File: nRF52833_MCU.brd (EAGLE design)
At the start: 51.3 x 30.2 mm, 64 parts, among them IC1 SKY13415-485LF, J1 282834-2, J100 DEBUG_CONNECTOR, J2 282834-2, J3 282834-2, U1 nRF52833-QIAA, U3 BQ25570RGRR, X1 32MHz, X2 32.768kHz, X3 22-23-2031

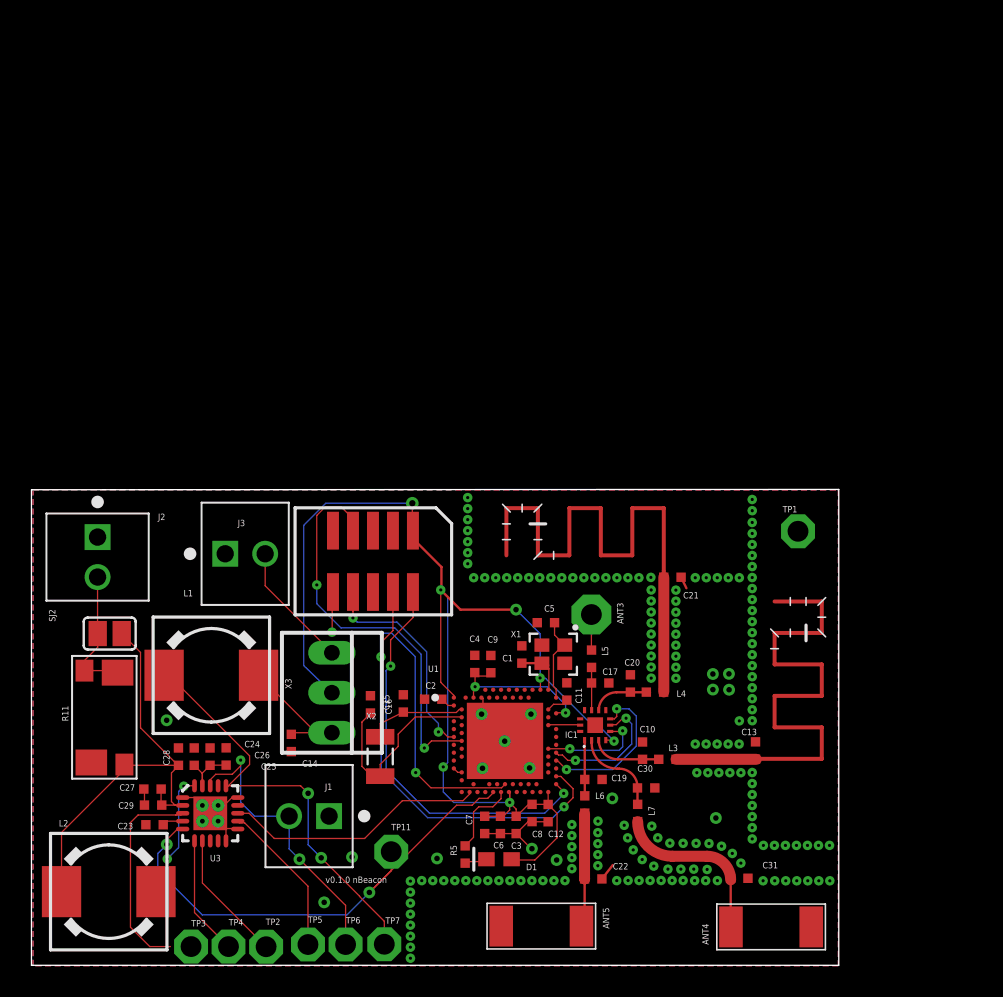
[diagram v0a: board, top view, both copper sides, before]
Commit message: Fix warnings
Signed-off-by: Florian Depraz <florian.depraz@outlook.com>
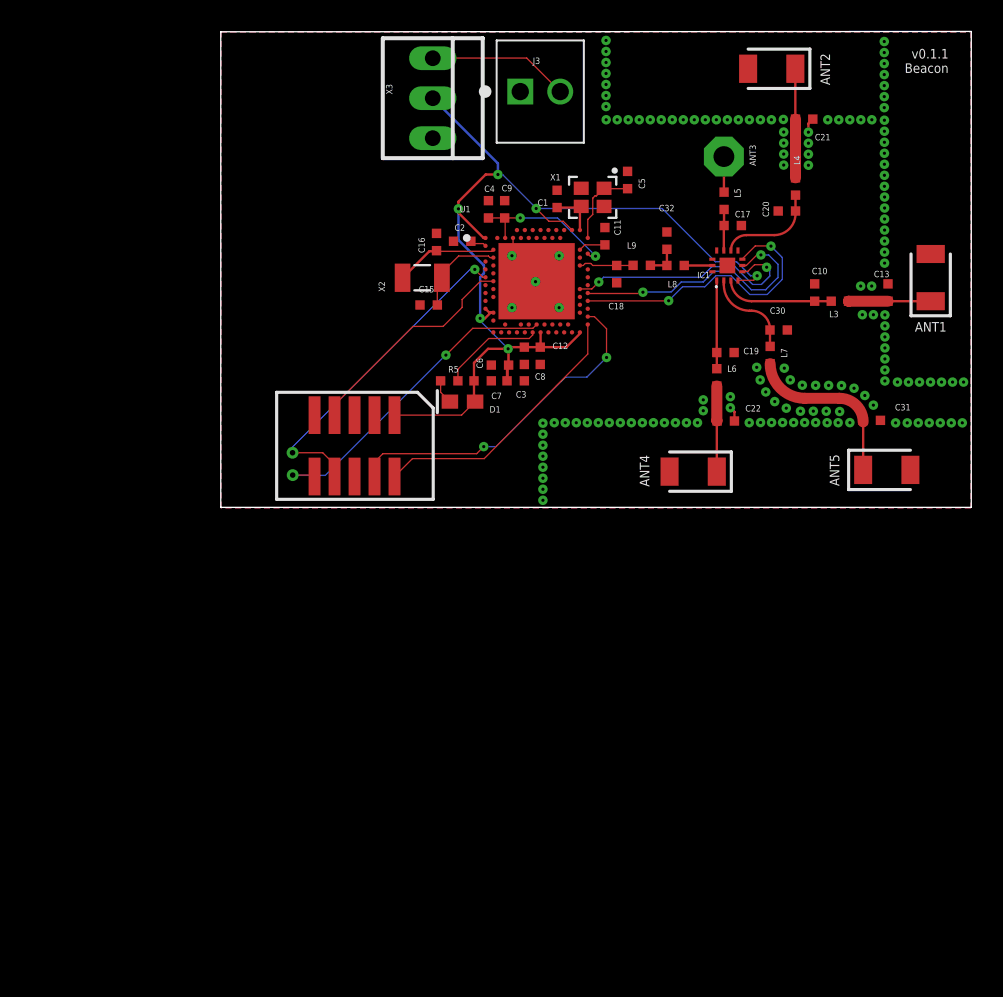
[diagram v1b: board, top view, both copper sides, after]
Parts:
- removed C14, C26, C29: NC, Nordic_misc:RESC0402_N
- removed C23: 0.01uF, Nordic_misc:RESC0402_N
- removed C24, C27: 0.1uF, Nordic_misc:RESC0402_N
- removed C25, C28: 4.7uF, Nordic_misc:RESC0402_N
- removed J1, J2: 282834-2, 282834-2:CONN_282834-2
- removed L1, L2: DR73-220-R, DR73-220-R:DR73
- removed R11: 0.05R, Y14870RXX000B9R:Y14870RXX000B9R
- removed SJ2: (no value), jumper:SJ
- removed TP1, TP11, TP2, TP3, TP4, TP5, TP6, TP7: TPPAD1-13, testpad:P1-13
- removed U3: BQ25570RGRR, BQ25570RGRR:QFN50P350X350X100-21N
- added C18: 1.0pF, Nordic_misc:RESC0402_N
- added C32: 1.2pF, Nordic_misc:RESC0402_N
- added L8: 2.2nH, Nordic_misc:RESC0402_N
- added L9: 4.7nH, Nordic_misc:RESC0402_N
- ANT1, ANT2: value (none) -> 2450AT18B100E; device Nordic_misc:QWMP_MEANDERED_LEFT_+6 -> 2450AT18B100E:ANTC3216X140N
- ANT4, ANT5: value SWRA092B -> 2450AT18B100E; device texas:SWRA092B -> 2450AT18B100E:ANTC3216X140N
- moved X3 38.3 mm to (28.5, 57.5)
- moved ANT5 36.4 mm to (57.3, 33.9), turned to 0 degrees
- moved J3 34.8 mm to (35.3, 57.9)
- moved L4 33.3 mm to (51.5, 51.9), turned to 90 degrees
- moved ANT2 32.6 mm to (50.0, 59.4), turned to 180 degrees
- moved ANT1 32.5 mm to (60.1, 46.1), turned to 90 degrees
- moved C20 31.6 mm to (51.0, 50.3), turned to 180 degrees
- moved L3 31.1 mm to (54.3, 44.6)
- moved C10 31.1 mm to (52.7, 45.2)
- moved X2 30.5 mm to (27.8, 46.1), turned to 0 degrees
- moved IC1 30.4 mm to (47.2, 46.9)
- moved C22 30.3 mm to (47.1, 37.0)
- moved C30 30.3 mm to (50.5, 42.8)
- moved L5 30.3 mm to (47.0, 51.0)
- moved ANT3 30.3 mm to (47.0, 53.8)
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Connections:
- removed net BQ_EXT_VBAT: J1.2, TP6.TP, U3.18
- removed net BQ_LBUCK: L1.2, TP7.TP, U3.16
- removed net BQ_NEN: TP11.TP, U1.AD10, U3.5
- removed net BQ_RSP1: J2.2, R11.P$3, R11.P$4, SJ2.2
- removed net BQ_SUPPLY_VBAT: C14.1, L1.1, X3.3
- removed net BQ_VBAT_OK: U1.AD4, U3.13
- removed net BQ_VBAT_OV: TP2.TP, U3.7
- removed net BQ_VIN_DC: C27.1, C28.1, C29.1, L2.1, R11.P$1, R11.P$2, SJ2.1, U3.2
- removed net BQ_VOUT: U3.14
- removed net BQ_VOUT_EN: TP4.TP, U3.6
- removed net BQ_VOUT_SET: TP5.TP, U3.12
- removed net BQ_VRDIV: U3.8
- removed net BQ_VSTOR: C24.1, C25.1, C26.1, U3.19
- removed net LBOOST: L2.2, U3.20
- removed net N$18: TP1.TP
- removed net VOC_SAMP: TP3.TP, U3.3
- removed net VREF_SAMP: C23.1, U3.4
- new net N$22: IC1.13, L8.2
- new net N$23: C32.1, L8.1, L9.2
- net GND: now also C18.2, C32.2; no longer C14.2, C23.2, C24.2, C25.2, C26.2, C27.2, C28.2, C29.2, J1.1, J2.1, U3.1, U3.10, U3.11, U3.15, U3.17, U3.21, U3.22, U3.23, U3.24, U3.25, U3.9
- net N$13: now also ANT4.1; no longer ANT5.1
- net N$14: now also ANT5.1; no longer ANT4.1
- net N$40: now also ANT2.1; no longer ANT2.P$1
- net N$5: now also ANT1.1; no longer ANT1.P$1
- net NRF_ANT: now also C18.1, L9.1; no longer IC1.13
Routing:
- net BQ_NEN: track 32.4 -> 0.00 mm, vias 2 -> 0
- net BQ_VIN_DC: track 28.6 -> 0.00 mm
- net BQ_LBUCK: track 27.2 -> 0.00 mm, vias 2 -> 0
- net BQ_EXT_VBAT: track 18.8 -> 0.00 mm, vias 2 -> 0
- net BQ_VBAT_OK: track 16.7 -> 0.00 mm
- net GND: track 16.9 -> 3.13 mm, vias 93 -> 39
- net VDD: track 82.5 -> 68.9 mm, vias 7 -> 6
- net VOC_SAMP: track 13.3 -> 0.00 mm
- net P0.07_RX: track 27.5 -> 14.3 mm, vias 2 -> 0
- net BQ_VOUT_SET: track 9.88 -> 0.00 mm
- net ANT_SEL_V3: track 6.69 -> 15.8 mm
- net BQ_SUPPLY_VBAT: track 8.79 -> 0.00 mm
- net ANT_SEL_V2: track 8.40 -> 17.1 mm
- net BQ_RSP1: track 8.45 -> 0.00 mm
- net BQ_VBAT_OV: track 8.41 -> 0.00 mm
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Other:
- board size 51.3 x 30.2 mm -> 47.7 x 30.2 mm
- board text added: "v0.1.1 Beacon"
- board text removed: "v0.1.0 nBeacon"
